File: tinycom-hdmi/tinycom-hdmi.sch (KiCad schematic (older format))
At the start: 42 parts, among them J1 MICRO_SD_HINGE, P1 CONN_02X10, P2 CONN_02X10, P4 USB_OTG, U1 SY8008BAAC, U2 AXP209, U3 SY8008BAAC, U4 RTL8188, U5 rainsun-antenna

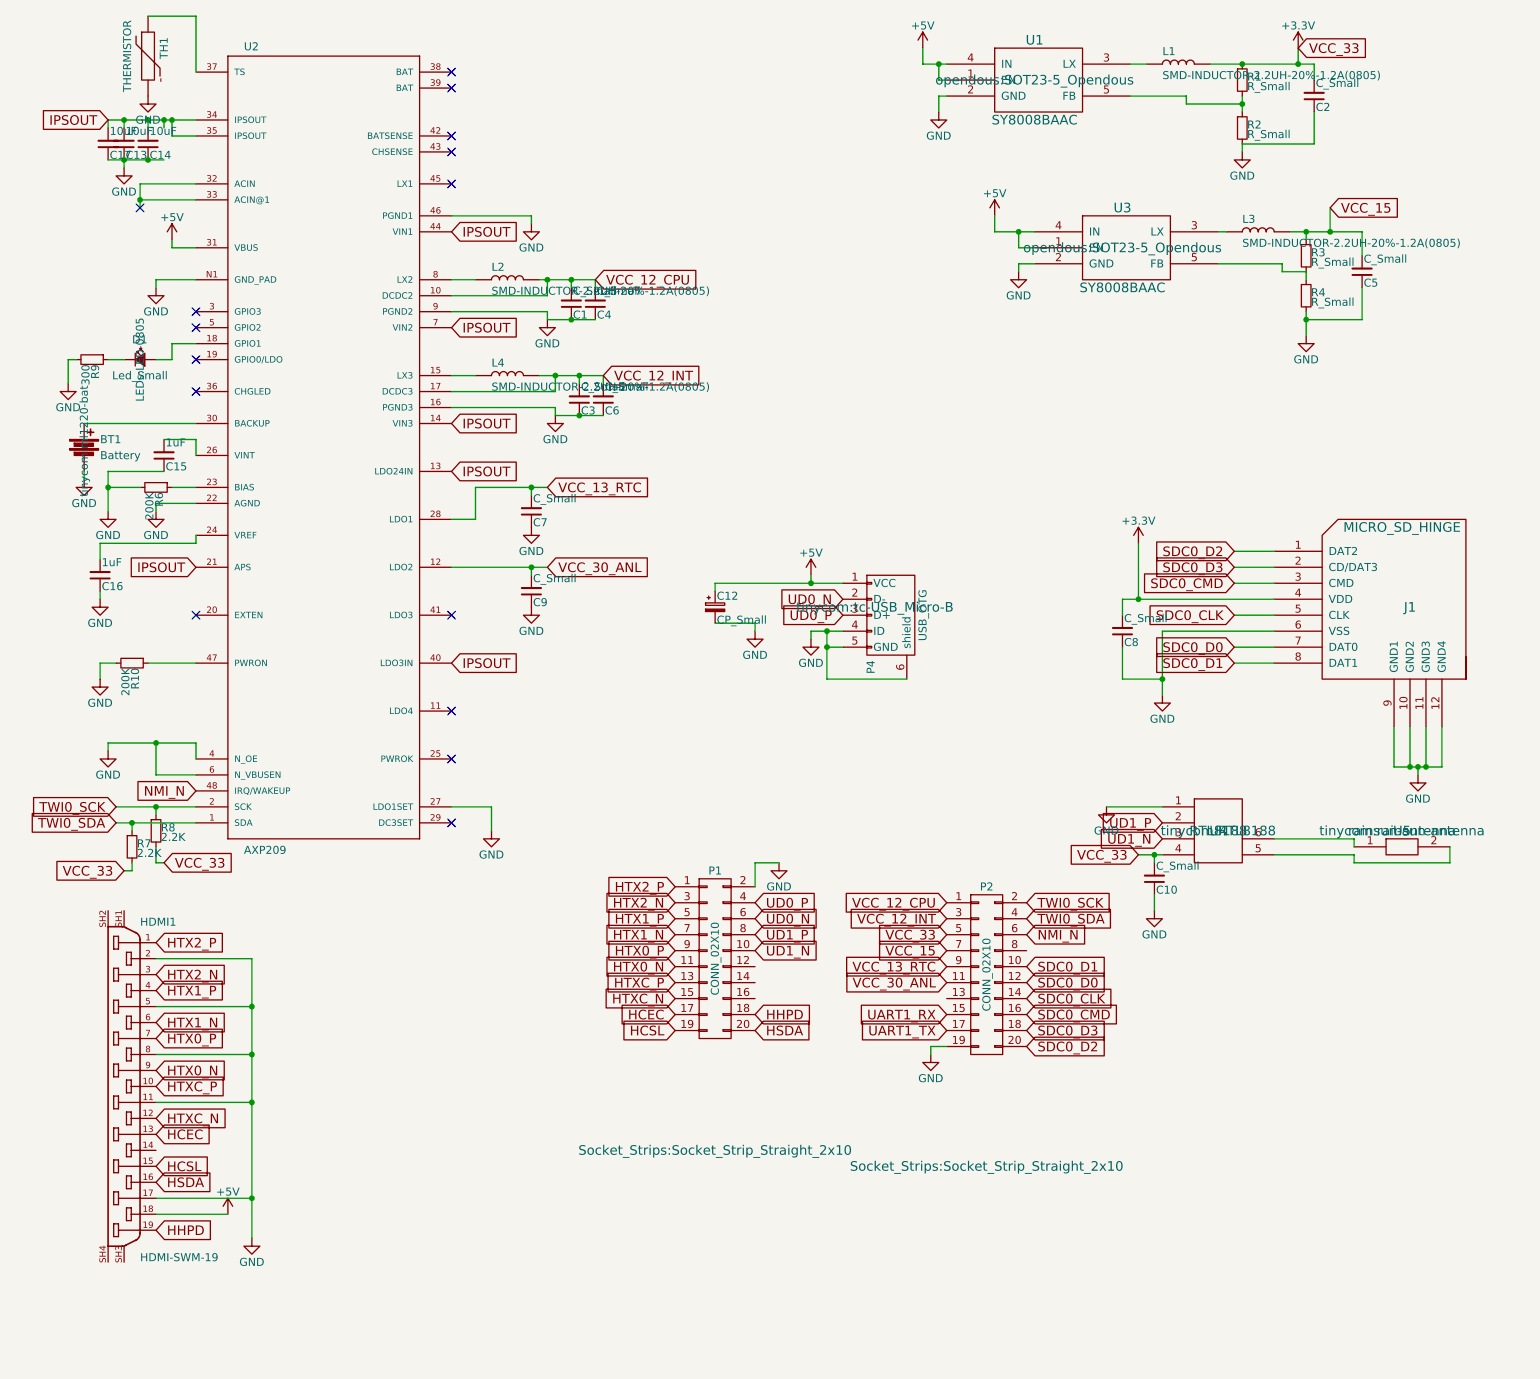
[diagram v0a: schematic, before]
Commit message: before replace
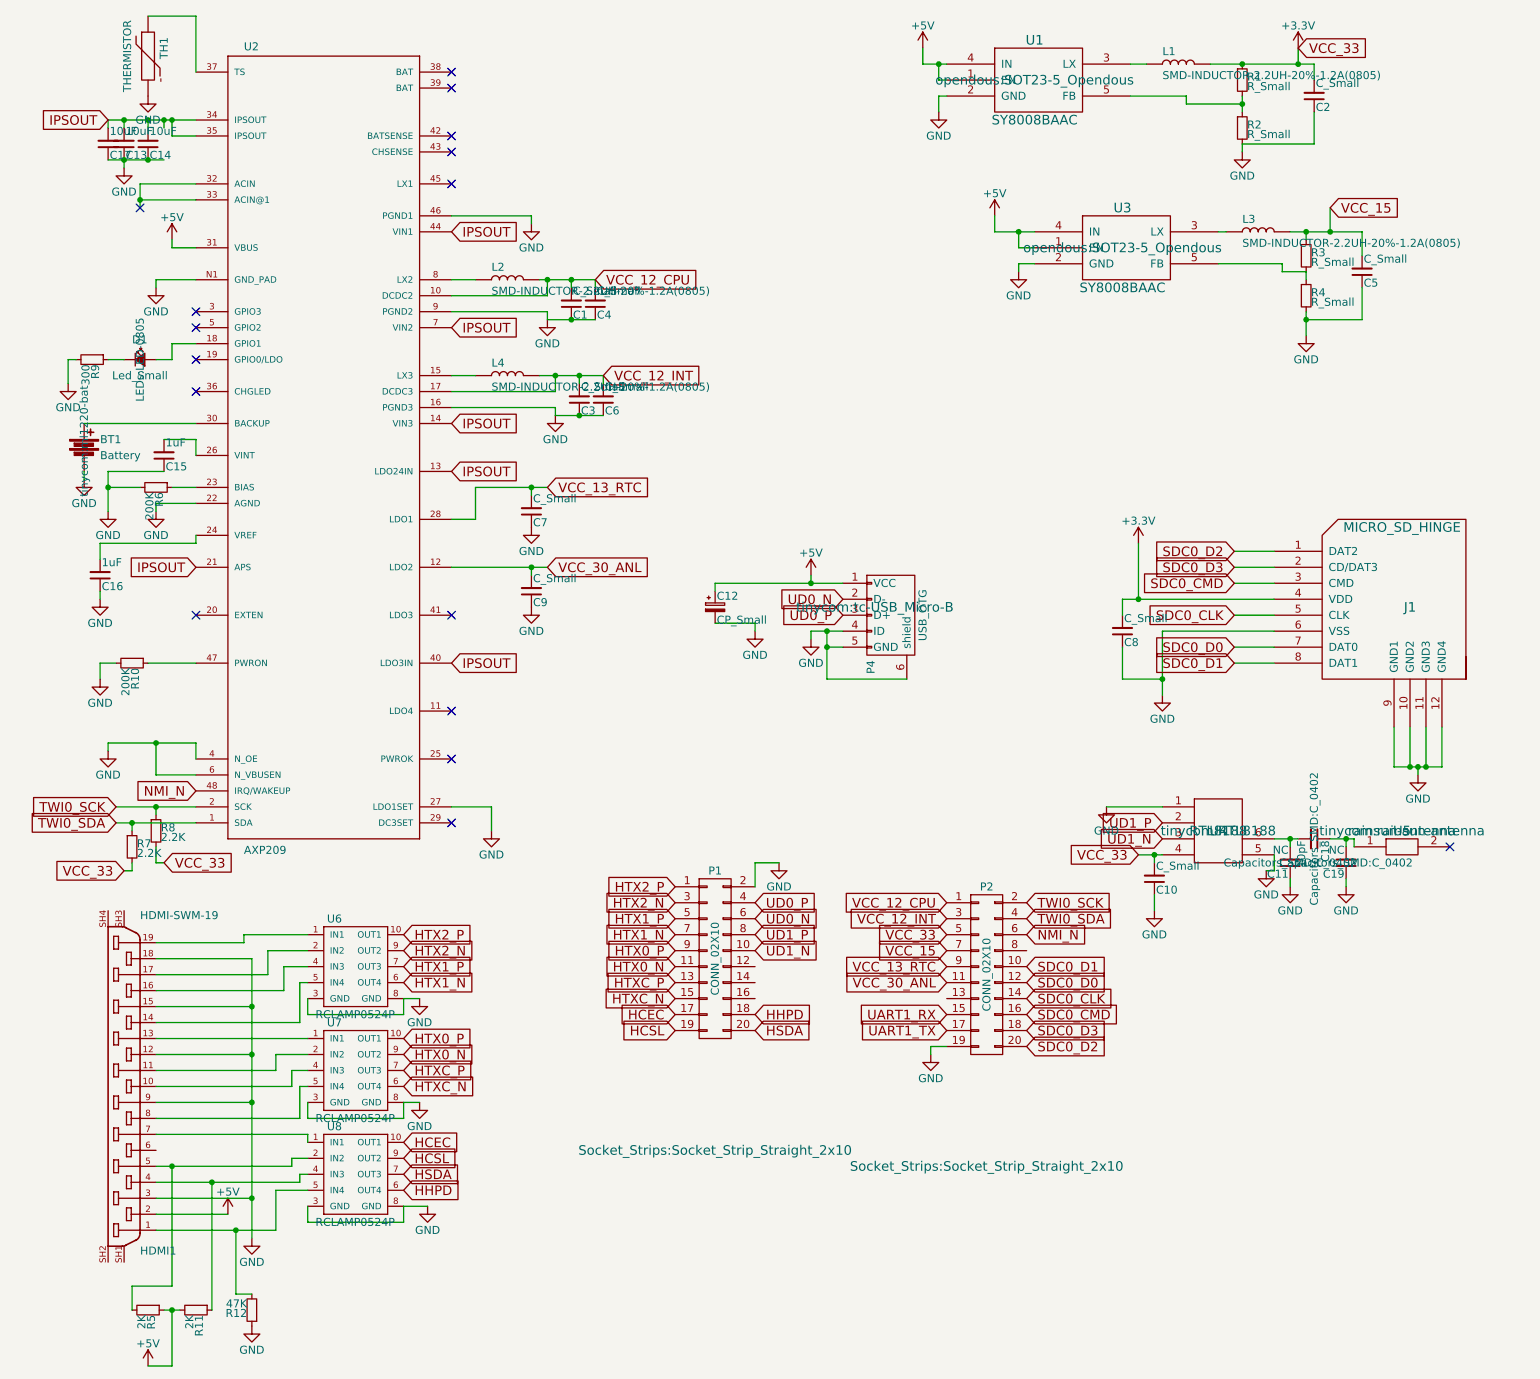
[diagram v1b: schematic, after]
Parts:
- added C11, C19: NC, Capacitors_SMD:C_0402, symbol C_Small
- added C18: 10pF, Capacitors_SMD:C_0402, symbol C_Small
- added R11, R5: 2K, Resistors_SMD:R_0805, symbol R_Small
- added R12: 47K, Resistors_SMD:R_0805, symbol R_Small
- added U6, U7, U8: RCLAMP0524P, tinycom:SLP2510P8, symbol RCLAMP0524P
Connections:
- net +5V: now also HDMI1.2, R11.2, R5.1; no longer HDMI1.18
- net GND: now also HDMI1.12, HDMI1.15, HDMI1.18, HDMI1.3, HDMI1.9, U4.5, C11.1, C19.1, R12.1, U6.3 (GND), U6.8 (GND), U7.3 (GND), U7.8 (GND), U8.3 (GND), U8.8 (GND); no longer HDMI1.11, HDMI1.17, HDMI1.2, HDMI1.5, HDMI1.8
- net HCEC: now also U8.10 (OUT1); no longer HDMI1.13
- net HCSL: now also U8.9 (OUT2); no longer HDMI1.15
- net HHPD: now also U8.6 (OUT4); no longer HDMI1.19
- net HSDA: now also U8.7 (OUT3); no longer HDMI1.16
- net HTX0_N: now also U7.9 (OUT2); no longer HDMI1.9
- net HTX0_P: now also U7.10 (OUT1); no longer HDMI1.7
- net HTX1_N: now also U6.6 (OUT4); no longer HDMI1.6
- net HTX1_P: now also U6.7 (OUT3); no longer HDMI1.4
- net HTX2_N: now also U6.9 (OUT2); no longer HDMI1.3
- net HTX2_P: now also U6.10 (OUT1); no longer HDMI1.1
- net HTXC_N: now also U7.6 (OUT4); no longer HDMI1.12
- net HTXC_P: now also U7.7 (OUT3); no longer HDMI1.10
- net at U5.2: no longer U4.5
- net at U4.6: now also C11.2, C18.2; no longer U5.1
- net at HDMI1.14: now also U6.5 (IN4)
- new net: C18.1, C19.2, U5.1
- new net: HDMI1.1, R12.2, U8.5 (IN4)
- new net: HDMI1.10, U7.4 (IN3)
- new net: HDMI1.11, U7.2 (IN2)
- new net: HDMI1.13, U7.1 (IN1)
- new net: HDMI1.16, U6.4 (IN3)
- new net: HDMI1.17, U6.2 (IN2)
- new net: HDMI1.19, U6.1 (IN1)
- new net: HDMI1.4, R11.1, U8.4 (IN3)
- new net: HDMI1.5, R5.2, U8.2 (IN2)
- new net: HDMI1.7, U8.1 (IN1)
- new net: HDMI1.8, U7.5 (IN4)
- no-connect marks 15 -> 16
